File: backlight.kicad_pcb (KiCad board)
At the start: 2 copper layers, 150 x 90 mm, 52 parts, among them J1 Screw_Terminal_01x03, U1 SY7203

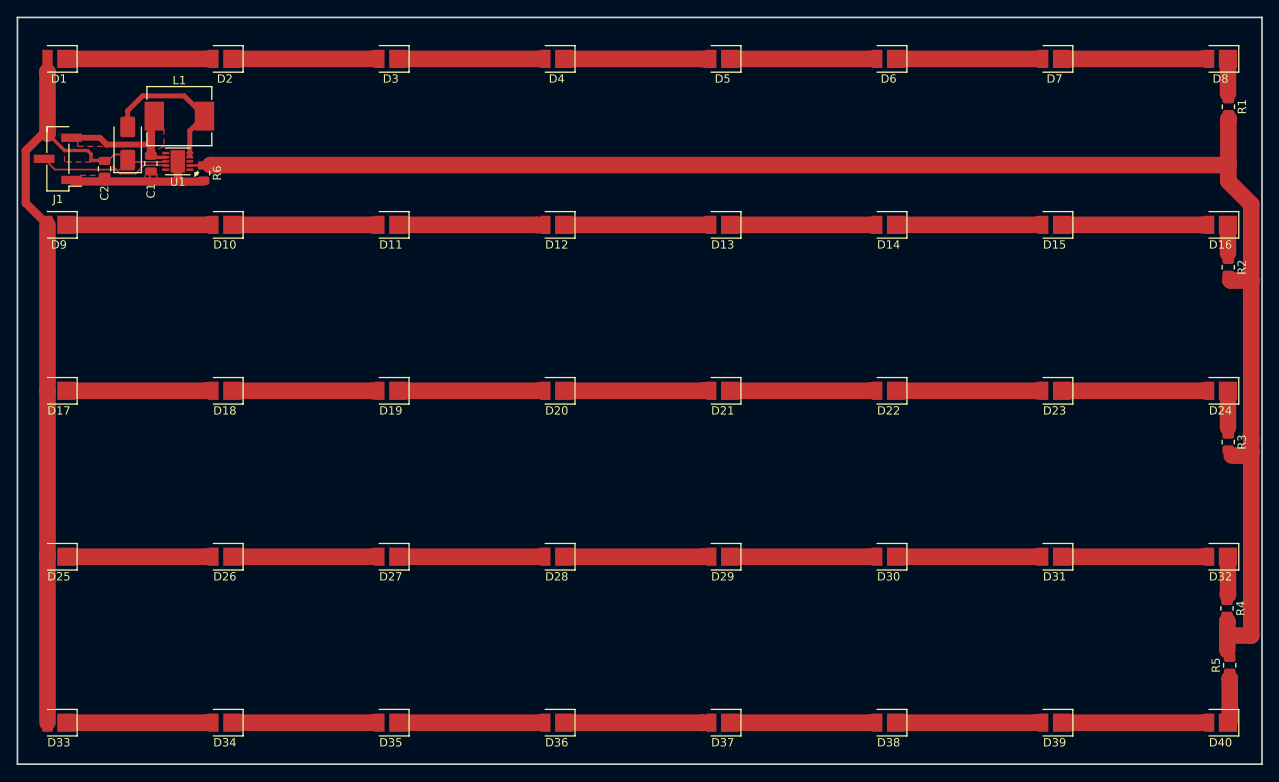
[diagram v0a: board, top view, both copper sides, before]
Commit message: Reroute board
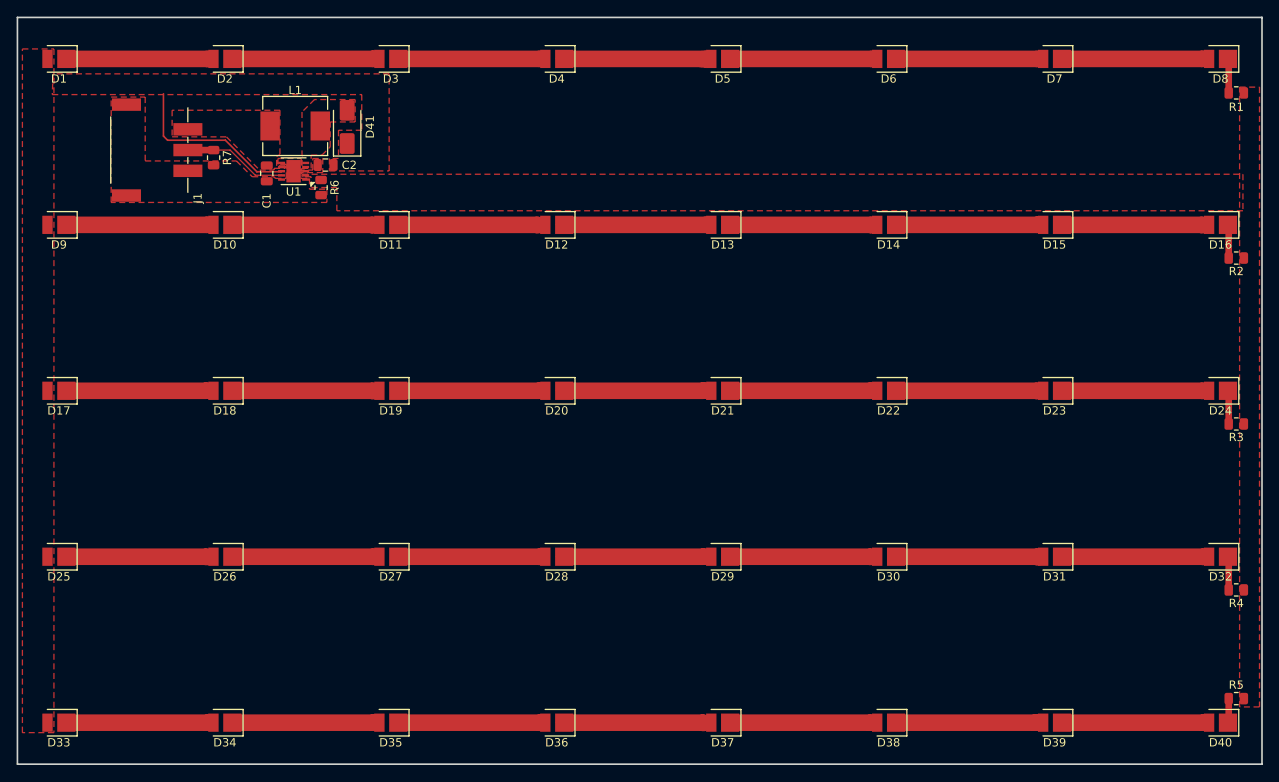
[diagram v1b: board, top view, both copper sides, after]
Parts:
- added R7: 10k, Resistor_SMD:R_0805_2012Metric, F.Cu at (68.6, 61.9)
- C1: value C -> 4.7uF 35V
- C2: value C -> 2.2uF 35V
- D41: value D_Schottky -> SS24
- J1: value Screw_Terminal_01x03 -> Conn_01x03_MountingPin; footprint Connector_PinHeader_2.54mm:PinHeader_1x03_P2.54mm_Vertical_SMD_Pin1Left -> rainwalker:XH254-0,5-3-2,5-V-SMD_1x03-1MP_P2.50mm_Vertical
- R6: value R -> 2R
- U1: footprint Package_DFN_QFN:DFN-10-1EP_3x3mm_P0.5mm_EP1.75x2.7mm -> rainwalker:SY7203DBC-DFN-10-1EP_3x3mm_P0.5mm_EP1.75x2.7mm
- moved C2 26.6 mm to (82.1, 62.8), turned to 180 degrees
- moved D41 26.5 mm to (84.7, 58.2)
- moved R6 14.3 mm to (81.6, 65.5)
- moved C1 14.0 mm to (75.0, 63.8)
- moved L1 14.0 mm to (78.5, 58.1)
- moved U1 14.0 mm to (78.3, 63.5)
- moved J1 12.0 mm to (61.8, 61.0), turned to 90 degrees
- moved R5 4.10 mm to (191.9, 127.1), turned to 0 degrees
- moved R4 2.49 mm to (191.9, 114.0), turned to 0 degrees
- moved R3 2.39 mm to (191.9, 94.0), turned to 0 degrees
- moved R1 1.91 mm to (191.9, 54.1), turned to 0 degrees
- moved R2 1.48 mm to (191.9, 74.0), turned to 0 degrees
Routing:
- net /LED-: track 200.6 -> 0.00 mm
- net /LED+: track 97.4 -> 21.1 mm
- net GND: track 19.9 -> 0.00 mm
- net Net-(D41-A): track 18.4 -> 0.00 mm
- net VPP: track 16.7 -> 0.00 mm
- net /EN_PWM: track 15.9 -> 12.6 mm
- net Net-(D40-K): track 6.60 -> 4.42 mm
- net Net-(D32-K): track 5.89 -> 4.04 mm
- net Net-(D16-K): track 3.43 -> 4.04 mm
- added copper zone on F.Cu, net /LED-
- added copper zone on F.Cu, net Net-(D41-A)
